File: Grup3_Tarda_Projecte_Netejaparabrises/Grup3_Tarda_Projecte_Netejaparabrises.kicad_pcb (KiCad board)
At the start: 4 copper layers, 162.4 x 126.4 mm, 92 parts, among them IC1 L78S05CV, IC2 PIC18F258-I_SO, J1 Screw_Terminal_01x02, J10 Screw_Terminal_01x02, J11 Screw_Terminal_01x02, J12 Screw_Terminal_01x02, J2 BOTONERA, J3 PROGRAMMING CON, J4 JP1, J5 DE9_Plug_MountingHoles, J6 DE9_Plug_MountingHoles, J7 CONEXIOSENSOR, J8 Screw_Terminal_01x02, J9 Screw_Terminal_01x02, K1 1393280-6, K2 1393280-6, K3 1393280-6, K4 1393280-6, K5 1393280-6, K6 1393280-6, K7 1393280-6, K8 1393280-6, K9 1393280-6, Q1 BC817-25_RF, Q2 BC817-25_RF, Q3 BC817-25_RF, Q4 BC817-25_RF, Q5 BC817-25_RF, Q6 BC817-25_RF, Q7 BC817-25_RF, SW1 SW_SPST, SW2 SW_SP3T, U1 Value, U2 LM393, Y1 ABLS2-8.000MHZ-D4Y-T

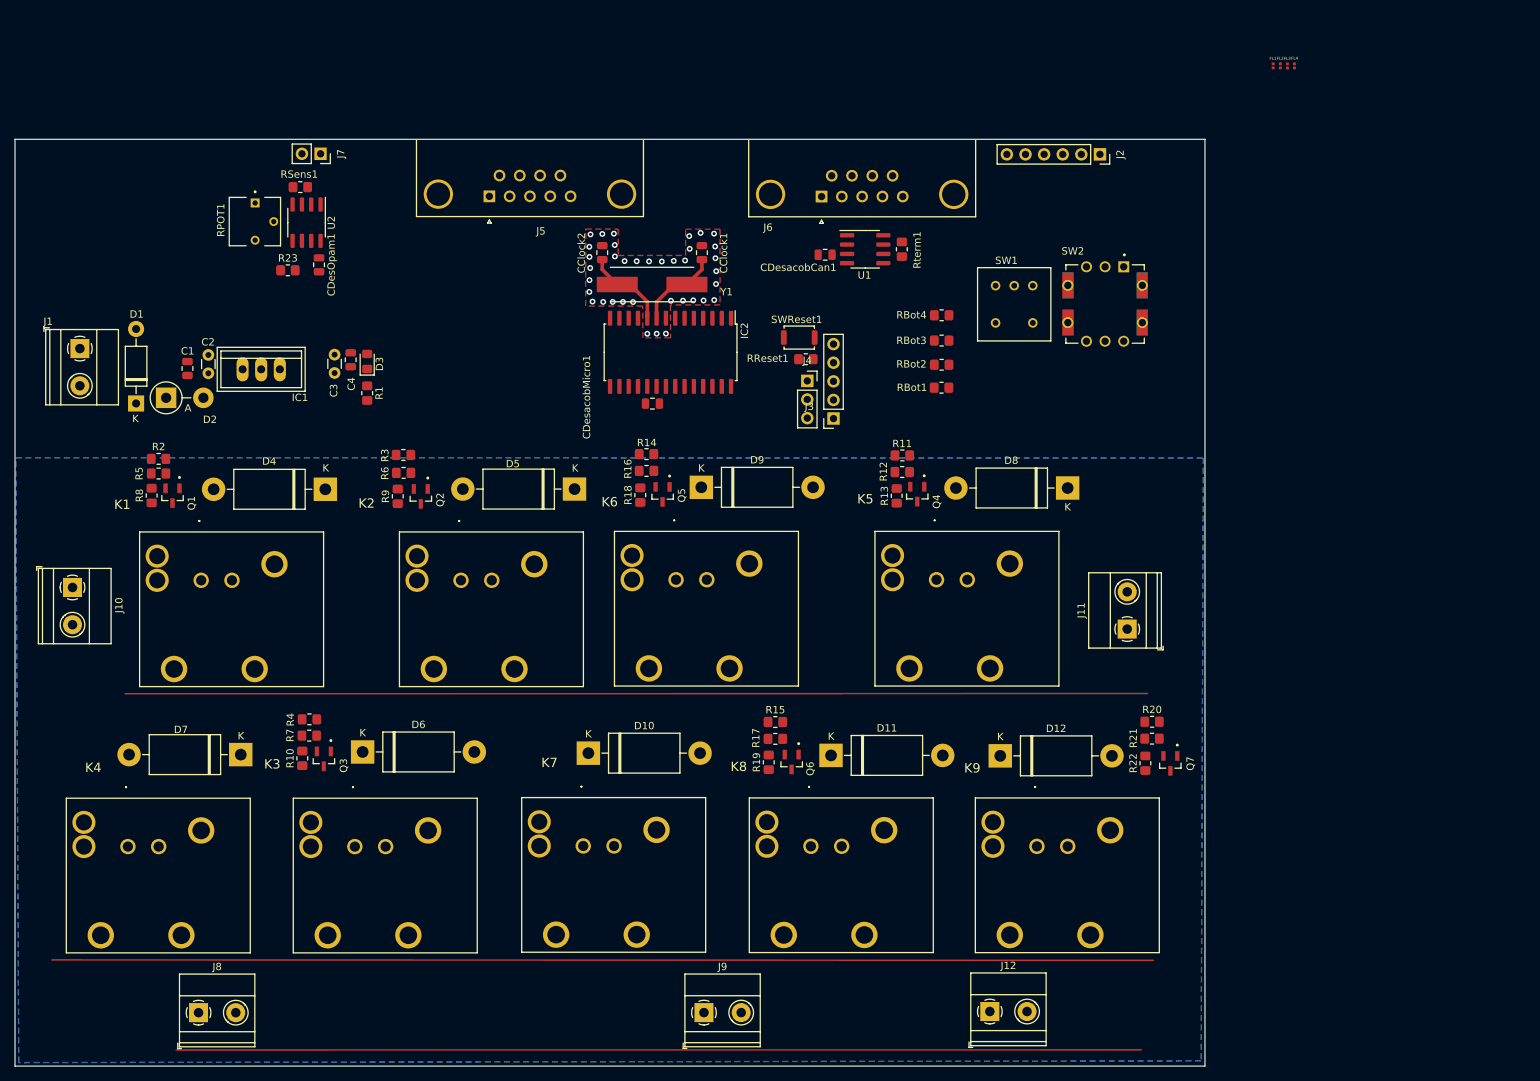
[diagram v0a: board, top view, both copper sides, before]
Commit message: routing v1 sense acabar
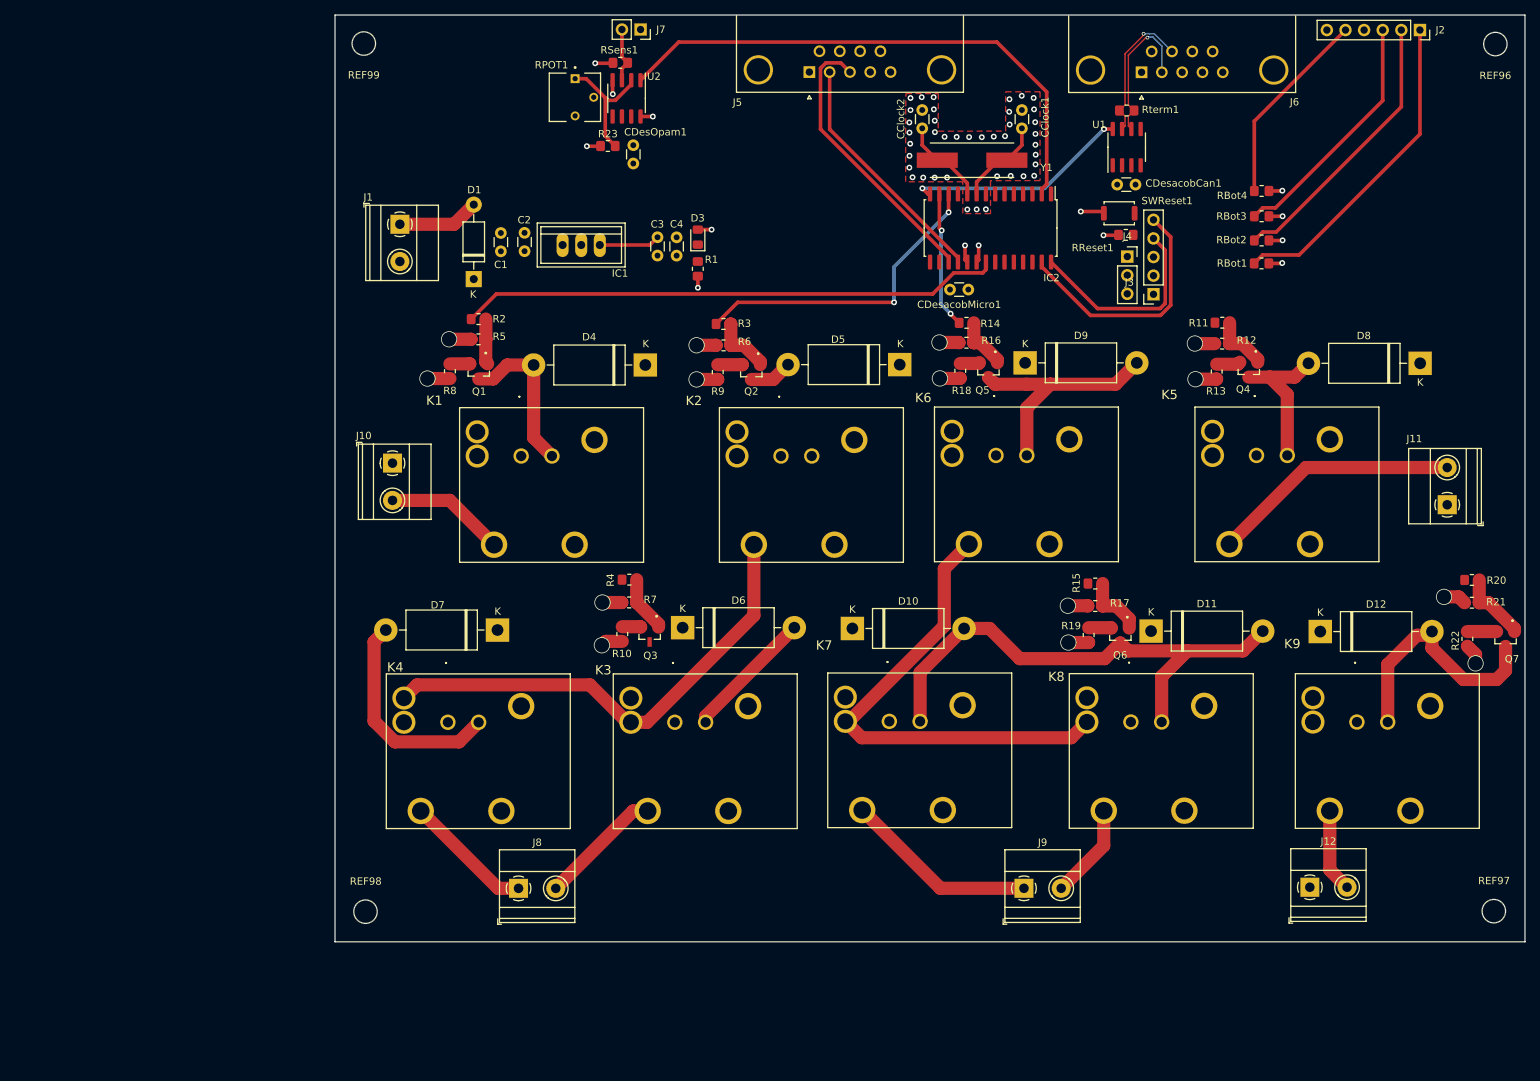
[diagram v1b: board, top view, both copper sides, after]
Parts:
- removed D2: 35V, Diode_THT:D_5W_P5.08mm_Vertical_AnodeUp
- removed FL1, FL2, FL3, FL4: BLM03HD331SZ1D, BLM03HD331SZ1D:BEADC0603X33N
- removed SW1: SW_SPST, Library:AS11CH
- removed SW2: SW_SP3T, SW_NR01103ANG13-1C:SW_NR01103ANG13-1C
- added REF96: MountingHole_3.2mm_M3_ISO7380, MountingHole:MountingHole_3.2mm_M3_ISO7380, F.Cu at (220.0, 36.8)
- added REF97: MountingHole_3.2mm_M3_ISO7380, MountingHole:MountingHole_3.2mm_M3_ISO7380, F.Cu at (219.8, 155.1)
- added REF98: MountingHole_3.2mm_M3_ISO7380, MountingHole:MountingHole_3.2mm_M3_ISO7380, F.Cu at (65.8, 155.1)
- added REF99: MountingHole_3.2mm_M3_ISO7380, MountingHole:MountingHole_3.2mm_M3_ISO7380, F.Cu at (65.6, 36.7)
- C1, C4, CClock1, CClock2, CDesOpam1, CDesacobCan1, CDesacobMicro1: footprint Capacitor_SMD:C_0805_2012Metric -> Capacitor_THT:C_Disc_D3.0mm_W1.6mm_P2.50mm
- moved D8 51.0 mm to (209.7, 80.3)
- moved D1 49.1 mm to (80.6, 68.8)
- moved Q7 48.8 mm to (221.4, 117.9)
- moved Q4 48.3 mm to (186.3, 81.2)
- moved D3 48.2 mm to (111.2, 63.1)
- moved R1 48.2 mm to (111.2, 67.4)
- moved Q2 48.2 mm to (118.5, 81.5)
- moved Q6 48.0 mm to (168.8, 117.5)
- moved R20 47.7 mm to (216.8, 109.9)
- moved R2 47.6 mm to (81.2, 74.3)
- moved R4 47.6 mm to (101.8, 109.8)
- moved Q5 47.6 mm to (150.8, 81.2)
- moved Q3 47.6 mm to (104.6, 117.3)
- moved R15 47.6 mm to (165.4, 110.4)
- moved D5 47.5 mm to (138.7, 80.5)
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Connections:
- net /Digital/CANH renamed /Digital/CAN-
- net /Digital/CANL renamed /Digital/CAN+
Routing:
- net Sensordig_o: track 0.00 -> 74.6 mm
- net DriverB1: track 0.00 -> 74.1 mm
- net /Potencia/Vc_m2: track 0.00 -> 71.2 mm
- net EN1: track 0.00 -> 66.3 mm
- net EN2: track 0.00 -> 66.2 mm
- net /Potencia/Vc_m1: track 0.00 -> 47.6 mm
- net /Digital/Vboto1: track 0.00 -> 44.1 mm
- net EnableM1: track 0.00 -> 43.4 mm, vias 0 -> 2
- net GNDPWR: track 0.00 -> 39.9 mm, vias 0 -> 14
- net /Digital/Tx: track 0.00 -> 38.5 mm
- net /Digital/Vboto2: track 0.00 -> 38.1 mm
- net PGC: track 0.00 -> 34.2 mm
- net VBOMBA2: track 0.00 -> 34.0 mm
- net /Digital/Vboto3: track 0.00 -> 33.7 mm
- net /Potencia/Vc_lu: track 0.00 -> 33.6 mm
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- removed copper zone on B.Cu, net GNDPWR
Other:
- board size 162.4 x 126.4 mm -> 162.4 x 126.5 mm
